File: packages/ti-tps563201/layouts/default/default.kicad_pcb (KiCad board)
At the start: 2 copper layers, 12 parts

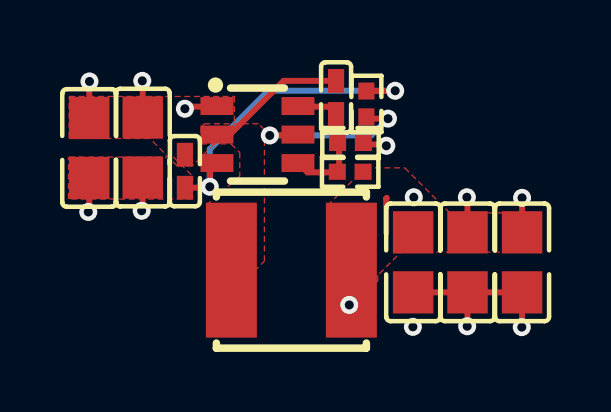
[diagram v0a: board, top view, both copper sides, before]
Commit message: layout tidy
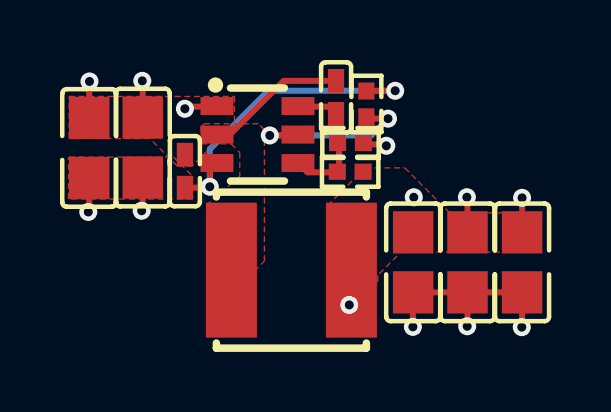
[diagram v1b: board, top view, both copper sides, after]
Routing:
- net power-VCC: track 3.51 -> 2.33 mm
- net GND: track 10.2 -> 11.4 mm
